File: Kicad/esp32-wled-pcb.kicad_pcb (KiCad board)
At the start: 2 copper layers, 25 parts, among them J1 Conn_01x03_Male, J2 Conn_01x03_Male, J4 Conn_01x02_Male, Q1 BS170F, SW1 SW_Push, SW2 SW_Push, U1 MT3420C, U2 ESP32-PICO-D4

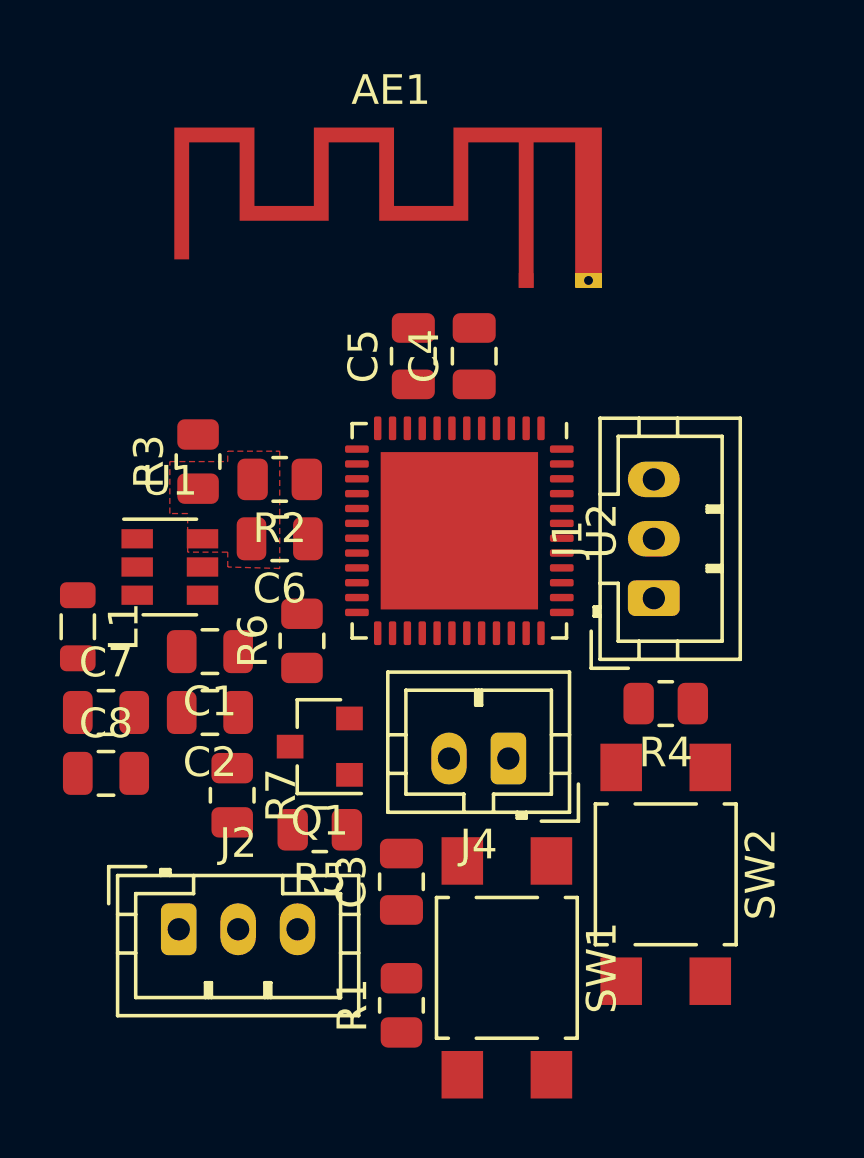
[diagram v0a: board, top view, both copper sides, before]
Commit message: still wip
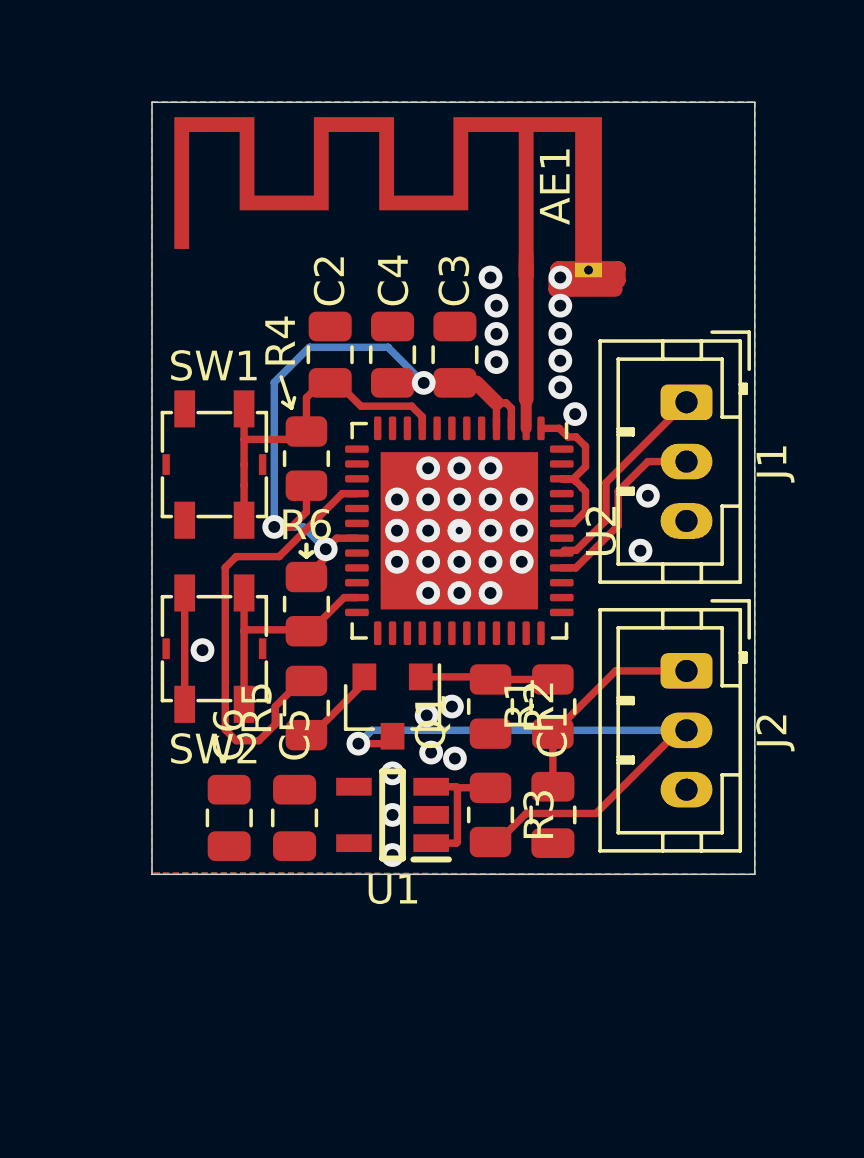
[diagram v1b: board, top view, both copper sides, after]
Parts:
- removed the C1 at (106.3, 63.6)
- removed the C6 at (108.7, 59.8)
- removed C7: C, Capacitor_SMD:C_0805_2012Metric
- removed J4: Conn_01x02_Male, Connector_JST:JST_PH_B2B-PH-K_1x02_P2.00mm_Vertical
- removed L1: L, Inductor_SMD:L_0805_2012Metric
- removed the R2 at (108.7, 57.8)
- removed the R3 at (106.0, 57.2)
- added C3: 10µ, Capacitor_SMD:C_0805_2012Metric, F.Cu at (114.6, 53.6)
- added R4: 4k7, Resistor_SMD:R_0805_2012Metric, F.Cu at (109.6, 57.1)
- C1: renamed from C2; value C -> 1µ
- C2: renamed from C3; value C -> 100n
- C4: value C -> 100n
- C5: value C -> 1µ
- C6: renamed from C8; value C -> 10µ
- R1: value R -> 4k7
- R5: value 4k7 -> 330R
- R6: renamed from R4; value R -> 4k7
- SW1, SW2: footprint Button_Switch_SMD:SW_SPST_TL3305B -> footprints:SW_XUNPU_TS-1077S
- U1: value MT3420C -> ME6211C33M5G; footprint Package_TO_SOT_SMD:SOT-23-6 -> footprints:SOT95P282X145-5N
- moved SW1 19.6 mm to (106.5, 57.3), turned to 90 degrees
- moved J2 19.2 mm to (122.4, 64.2), turned to 270 degrees
- moved C2 17.9 mm to (110.4, 53.6)
- moved SW2 17.0 mm to (106.5, 63.5), turned to 90 degrees
- moved C5 16.1 mm to (109.2, 69.2), turned to 270 degrees
- moved R6 12.6 mm to (109.6, 62.0), turned to 270 degrees
- moved C1 12.1 mm to (117.9, 69.1), turned to 270 degrees
- moved R1 11.3 mm to (117.9, 65.5)
- moved U1 11.2 mm to (112.5, 69.1), turned to 180 degrees
- moved R3 8.73 mm to (115.8, 69.1)
- moved R2 6.72 mm to (115.8, 65.5), turned to 270 degrees
- moved J1 6.69 mm to (122.4, 55.2), turned to 270 degrees
- moved C6 4.41 mm to (107.0, 69.2), turned to 270 degrees
- moved R5 4.12 mm to (109.6, 65.5), turned to 90 degrees
- moved Q1 2.80 mm to (112.5, 65.5), turned to 270 degrees
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- renumbered R6 to R2, R7 to R3
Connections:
- net /WLED_D1 renamed /LED_DATA
- J1 pad 1: GND -> /ESP32_TXD
- J1 pad 3: /ESP32_TXD -> GND
- J2 pad 1: GND -> +5V
- J2 pad 3: +5V -> GND
- Q1 pad 2: /ESP_IO27 -> Net-(Q1-Pad2)
- R1 pad 1: +3V3 -> +5V
- R1 pad 2: /RST -> Net-(Q1-Pad1)
- R5 pad 1: +5V -> Net-(Q1-Pad2)
- R5 pad 2: Net-(Q1-Pad1) -> Net-(R5-Pad2)
- U1 pad 3: Net-(L1-Pad1) -> +5V
- U1 pad 4: +5V -> (no net)
- U1 pad 5: (no net) -> +3V3
- U2 pad 16: /ESP_IO27 -> Net-(R5-Pad2)
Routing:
- net +3V3: track 0.00 -> 29.4 mm, vias 0 -> 3
- net /LED_DATA: track 0.00 -> 20.8 mm, vias 0 -> 1
- net Net-(R5-Pad2): track 0.00 -> 15.0 mm
- net /RST: track 0.00 -> 12.1 mm
- net +5V: track 0.00 -> 11.9 mm
- net GND: track 0.00 -> 11.7 mm, vias 0 -> 40
- net /BOOT: track 0.00 -> 8.05 mm
- net /ESP32_TXD: track 0.00 -> 7.05 mm
- net /ESP32_RXD: track 0.00 -> 6.36 mm
- net Net-(AE1-Pad1): track 0.00 -> 5.68 mm
- net Net-(Q1-Pad1): track 0.00 -> 4.49 mm
- net Net-(Q1-Pad2): track 0.00 -> 2.88 mm
- net (no net): vias 0 -> 1
- added copper zone on B.Cu, net GND
- added copper zone on F.Cu, net GND
- removed copper zone on F.Cu, net Net-(C6-Pad2)
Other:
- board outline added: 20.3 x 26 mm
- net class Default: clearance 0.2 -> 0.16
- rule trace_clearance: 0.2 -> 0.16

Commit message: finalize design
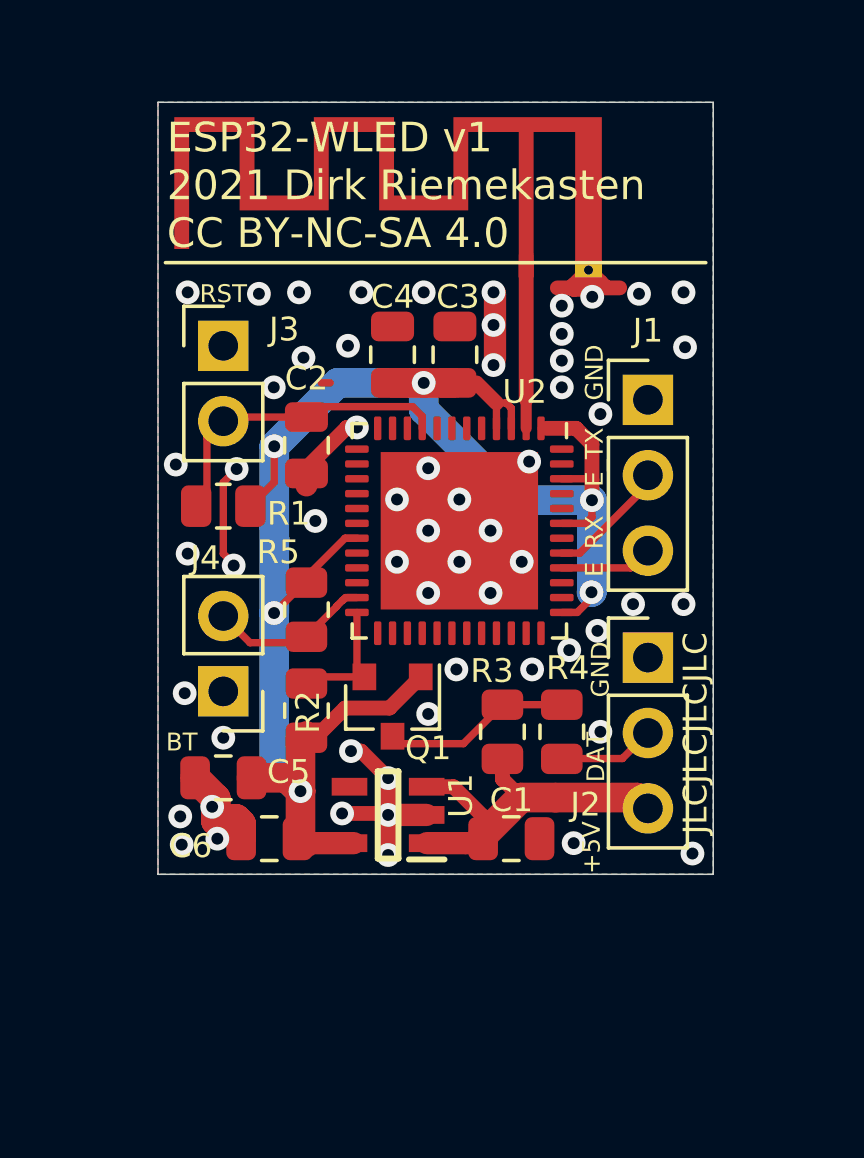
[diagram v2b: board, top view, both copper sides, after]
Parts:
- removed the R1 at (117.9, 65.5)
- removed the R5 at (109.6, 65.5)
- removed SW2: SW_Push, footprints:SW_XUNPU_TS-1077S
- added J4: SW_Push, Connector_PinHeader_2.54mm:PinHeader_1x02_P2.54mm_Vertical, F.Cu at (106.8, 64.9)
- added R4: 10R, Resistor_SMD:R_0805_2012Metric, F.Cu at (118.2, 66.3)
- J1, J2: footprint Connector_JST:JST_PH_B3B-PH-K_1x03_P2.00mm_Vertical -> Connector_PinHeader_2.54mm:PinHeader_1x03_P2.54mm_Vertical
- J3: renamed from SW1; footprint footprints:SW_XUNPU_TS-1077S -> Connector_PinHeader_2.54mm:PinHeader_1x02_P2.54mm_Vertical
- R2: value 10k -> 4k7
- moved R2 6.20 mm to (109.6, 65.6), turned to 90 degrees
- moved J3 4.01 mm to (106.8, 53.3), turned to 0 degrees
- moved R1 3.22 mm to (106.8, 58.7), turned to 180 degrees
- moved C2 3.15 mm to (109.6, 56.6), turned to 270 degrees
- moved R3 2.83 mm to (116.2, 66.3), turned to 90 degrees
- moved C5 2.75 mm to (106.8, 67.8), turned to 180 degrees
- moved C1 1.61 mm to (116.5, 69.9), turned to 0 degrees
- moved C6 1.52 mm to (108.3, 69.9), turned to 180 degrees
- moved J2 1.38 mm to (121.1, 63.8), turned to 0 degrees
- moved J1 1.30 mm to (121.1, 55.1), turned to 0 degrees
- moved R5 0.19 mm to (109.6, 62.2)
- moved U1 0.15 mm to (112.3, 69.1)
- renumbered R4 to R1, R6 to R5
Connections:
- J1 pad 1: /ESP32_TXD -> GND
- J1 pad 2: /ESP32_RXD -> /ESP32_TXD
- J1 pad 3: GND -> /ESP32_RXD
- J2 pad 1: +5V -> GND
- J2 pad 3: GND -> +5V
- Q1 pad 1: Net-(Q1-Pad1) -> +3V3
- Q1 pad 3: /LED_DATA -> Net-(Q1-Pad3)
- R2 pad 1: Net-(Q1-Pad1) -> +3V3
- R2 pad 2: GND -> Net-(Q1-Pad2)
- R3 pad 2: /LED_DATA -> Net-(Q1-Pad3)
- U2 pad 16: Net-(R5-Pad2) -> (no net)
- U2 pad 24: (no net) -> Net-(Q1-Pad2)
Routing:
- net +3V3: track 29.4 -> 62.0 mm, vias 3 -> 6
- net /LED_DATA: track 20.8 -> 3.26 mm, vias 1 -> 0
- net Net-(R5-Pad2): track 15.0 -> 0.00 mm
- net GND: track 11.7 -> 22.8 mm, vias 40 -> 58
- net Net-(Q1-Pad3): track 0.00 -> 6.35 mm
- net Net-(Q1-Pad1): track 4.49 -> 0.00 mm
- net /ESP32_RXD: track 6.36 -> 3.14 mm
- net /ESP32_TXD: track 7.05 -> 4.18 mm
- net /BOOT: track 8.05 -> 5.51 mm
- net Net-(Q1-Pad2): track 2.88 -> 4.24 mm
- net +5V: track 11.9 -> 13.1 mm
- net /RST: track 12.1 -> 11.1 mm
- net (no net): vias 1 -> 0
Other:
- board size 20.3 x 26 mm -> 18.7 x 26 mm
- board text added: "+5V"
- board text added: "BT"
- board text added: "DAT"
- board text added: "ESP32-WLED v1 2021 Dirk Riemekasten CC BY-NC-SA 4.0"
- board text added: "E_RX"
- board text added: "E_TX"
- board text added: "GND"
- board text added: "JLCJLCJLCJLC"
- board text added: "RST"
